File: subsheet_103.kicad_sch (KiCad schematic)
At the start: 28 parts, among them J5 DB25 Parallel Port, Q1 2N3904, U19 YM2149, U40 QUAD 2-INPUT NOR GATES

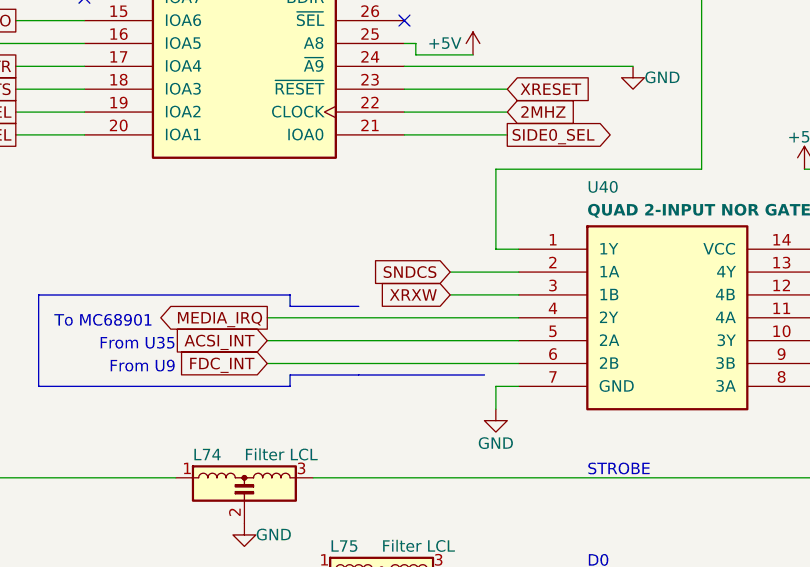
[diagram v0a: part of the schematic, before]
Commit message: fixed U40 -- pin 2 and 3 were switched
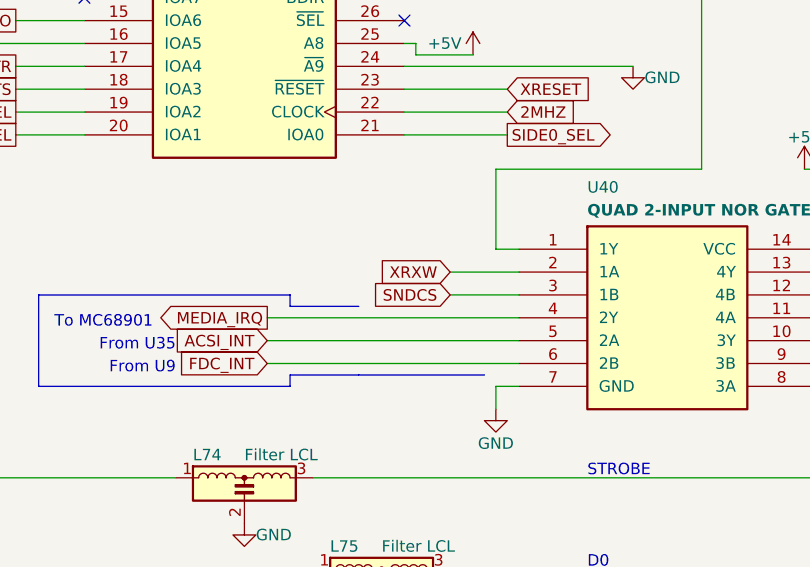
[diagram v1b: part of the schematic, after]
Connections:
- net SNDCS: now also U40.3 (1B); no longer U40.2 (1A)
- net XRXW: now also U40.2 (1A); no longer U40.3 (1B)
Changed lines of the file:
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@@
     )
   )
-  (global_label "XRXW" (shape input) (at 124.46 129.54 180) (fields_autoplaced)
+  (global_label "XRXW" (shape input) (at 124.46 127 180) (fields_autoplaced)
     (effects (font (size 1.27 1.27)) (justify right))
-    (property "Intersheetrefs" "${INTERSHEET_REFS}" (at 116.9953 129.4606 0)
+    (property "Intersheetrefs" "${INTERSHEET_REFS}" (at 116.9953 126.9206 0)
       (effects (font (size 1.27 1.27)) (justify right) hide)
     )
@@
     )
   )
-  (global_label "SNDCS" (shape input) (at 124.46 127 180) (fields_autoplaced)
+  (global_label "SNDCS" (shape input) (at 124.46 129.54 180) (fields_autoplaced)
     (effects (font (size 1.27 1.27)) (justify right))
-    (property "Intersheetrefs" "${INTERSHEET_REFS}" (at 115.8463 126.9206 0)
+    (property "Intersheetrefs" "${INTERSHEET_REFS}" (at 115.8463 129.4606 0)
       (effects (font (size 1.27 1.27)) (justify right) hide)
     )
